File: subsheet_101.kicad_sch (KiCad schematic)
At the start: 5 parts

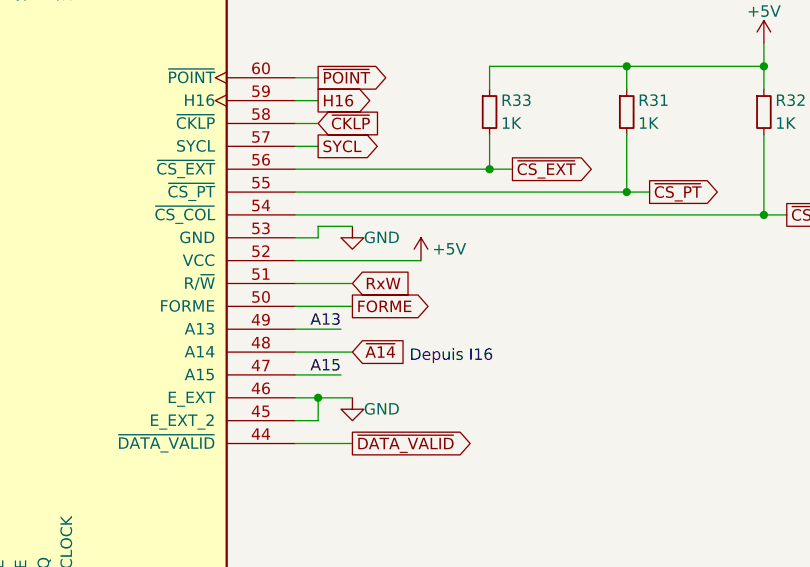
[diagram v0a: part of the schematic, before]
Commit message: commence PIA
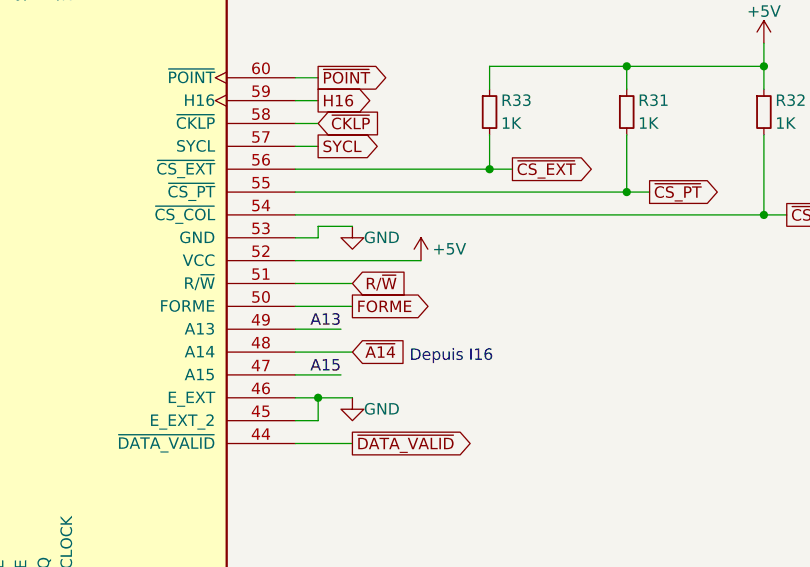
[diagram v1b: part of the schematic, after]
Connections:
- net RxW renamed R/~{W}
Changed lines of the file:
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@@
     )
   )
-  (global_label "RxW" (shape input) (at 132.08 116.84 0) (fields_autoplaced)
+  (global_label "R{slash}~{W}" (shape input) (at 132.08 116.84 0) (fields_autoplaced)
     (effects (font (size 1.27 1.27)) (justify left))
-    (property "Intersheet References" "${INTERSHEET_REFS}" (id 0) (at 138.2426 116.7606 0)
+    (property "Intersheet References" "${INTERSHEET_REFS}" (id 0) (at 138.545 116.7606 0)
       (effects (font (size 1.27 1.27)) (justify left) hide)
     )
